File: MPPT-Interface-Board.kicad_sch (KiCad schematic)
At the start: 13 parts, among them J1 MPPT CAN 1, J2 MPPT CAN 2, J3 CarCAN 1, J4 CarCAN 2, J5 FUSEBOX, J6 CANDAPTER, U1 RI3-1209S

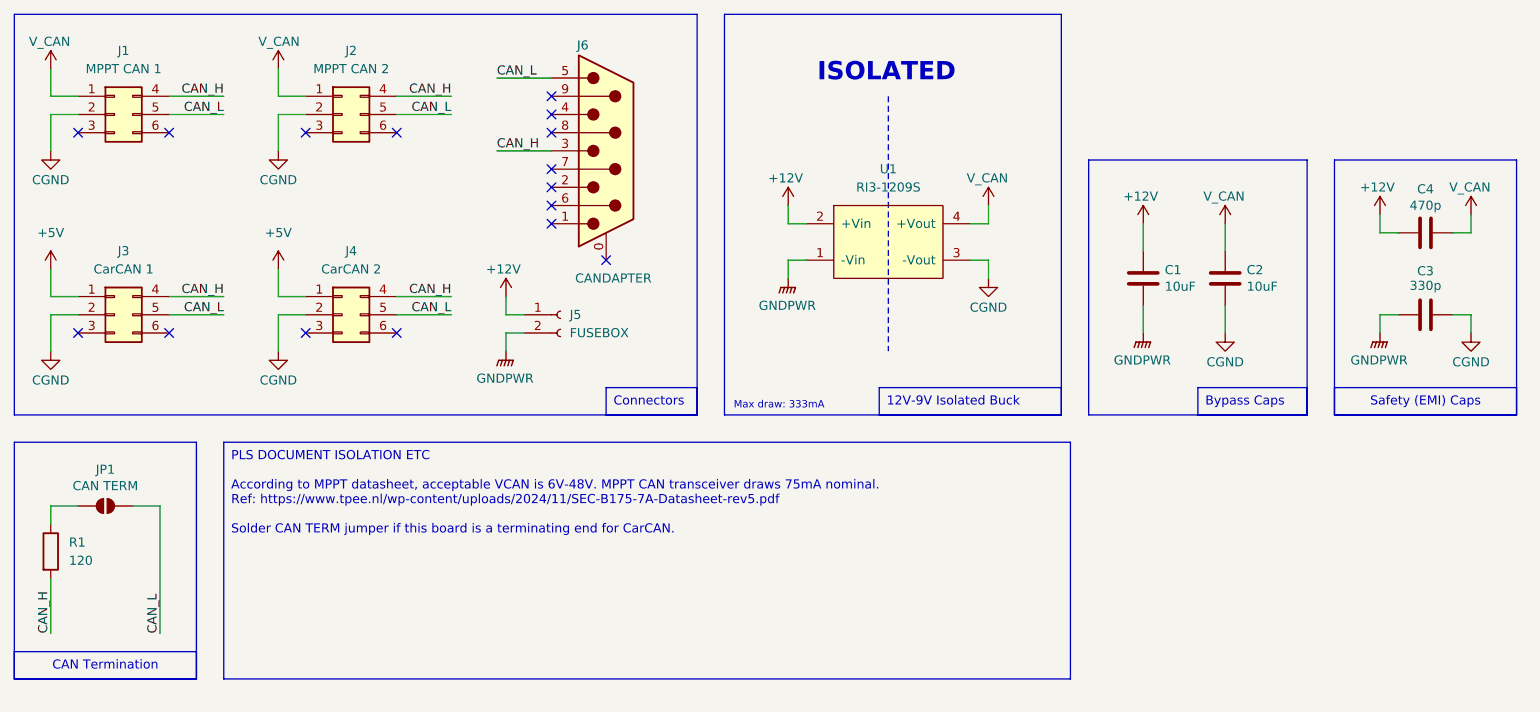
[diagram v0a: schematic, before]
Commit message: add RPP
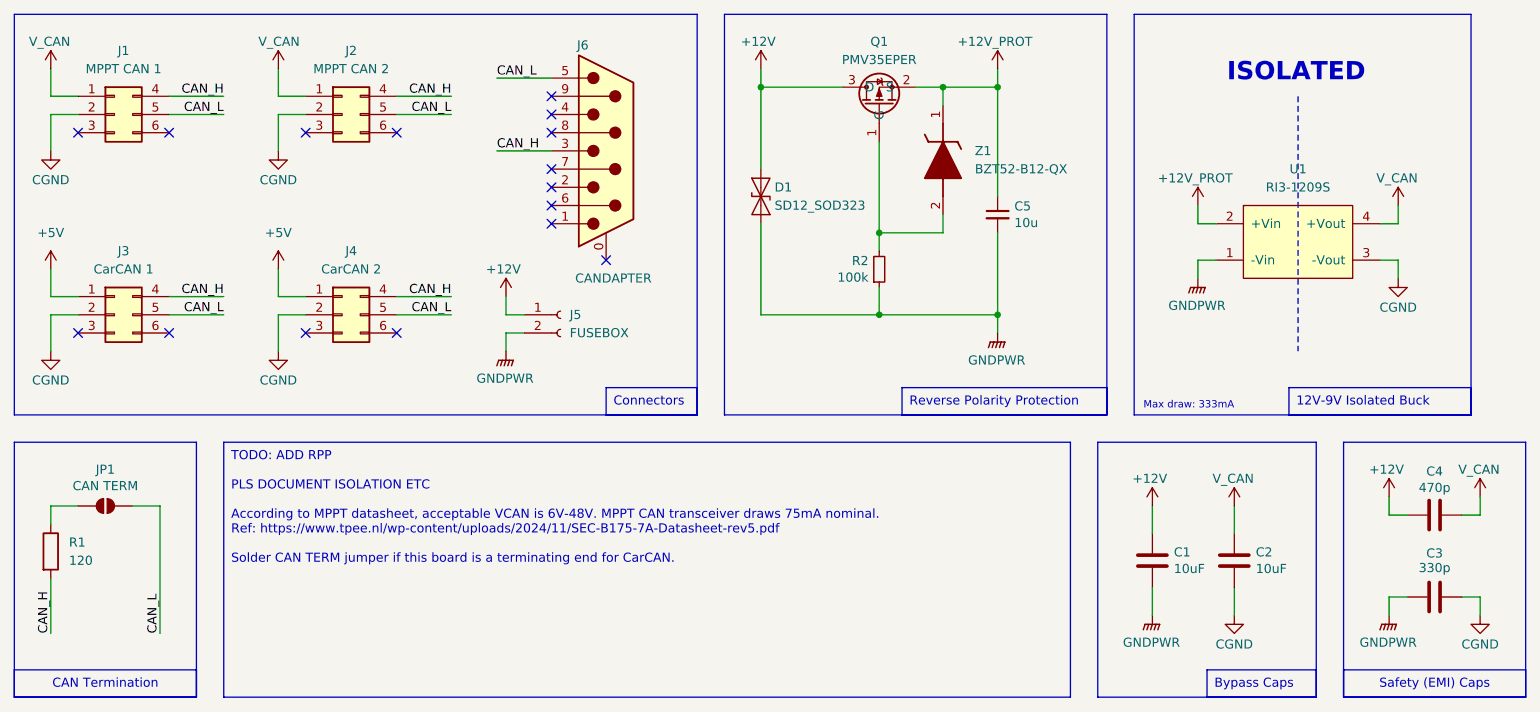
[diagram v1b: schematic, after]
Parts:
- added C5: 10u, Capacitor_SMD:C_0805_2012Metric, symbol Device:C_Small
- added D1: SD12_SOD323, Diode_SMD:D_SOD-323, symbol Diode:SD12_SOD323
- added Q1: PMV35EPER, Package_TO_SOT_SMD:SOT-23, symbol utsvt-chips:PMV35EPE
- added R2: 100k, Resistor_SMD:R_0805_2012Metric, symbol Device:R_Small
- added Z1: BZT52-B12-QX, Zener:BZT52B12QX, symbol BZT52-B12-QX:BZT52-B12-QX
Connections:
- net +12V: now also D1.2 (A2), Q1.3 (D); no longer U1.2 (+Vin)
- net GNDPWR: now also C5.2, D1.1 (A1), R2.1
- new net: Q1.1 (G), R2.2, Z1.2 (A)
- new net +12V_PROT: C5.1, Q1.2 (S), U1.2 (+Vin), Z1.1 (K)
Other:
- moved on the sheet: C1, C2, C3, C4, U1
